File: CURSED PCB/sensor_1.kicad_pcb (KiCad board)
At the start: 4 copper layers, 42 x 40 mm, 85 parts, among them J1 Debugging Connector, J2 Micro_SD_Card, J3 Gecko Connector, J5 G125-MH104M4-04AD000P, U1 STM32G431KBT6, U10 MCP2562, U12 AD5761BRUZ, U2 INA180-A3, U3 MIC94090YC6, U4 SPX3819M5-L-3-3, U5 SPX3819M5-L-3-3, U6 OPA323, U7 MCP3562-E_ST, U8 LT6233, U9 TLV61046ADBVR, Y1 24MHz crystal

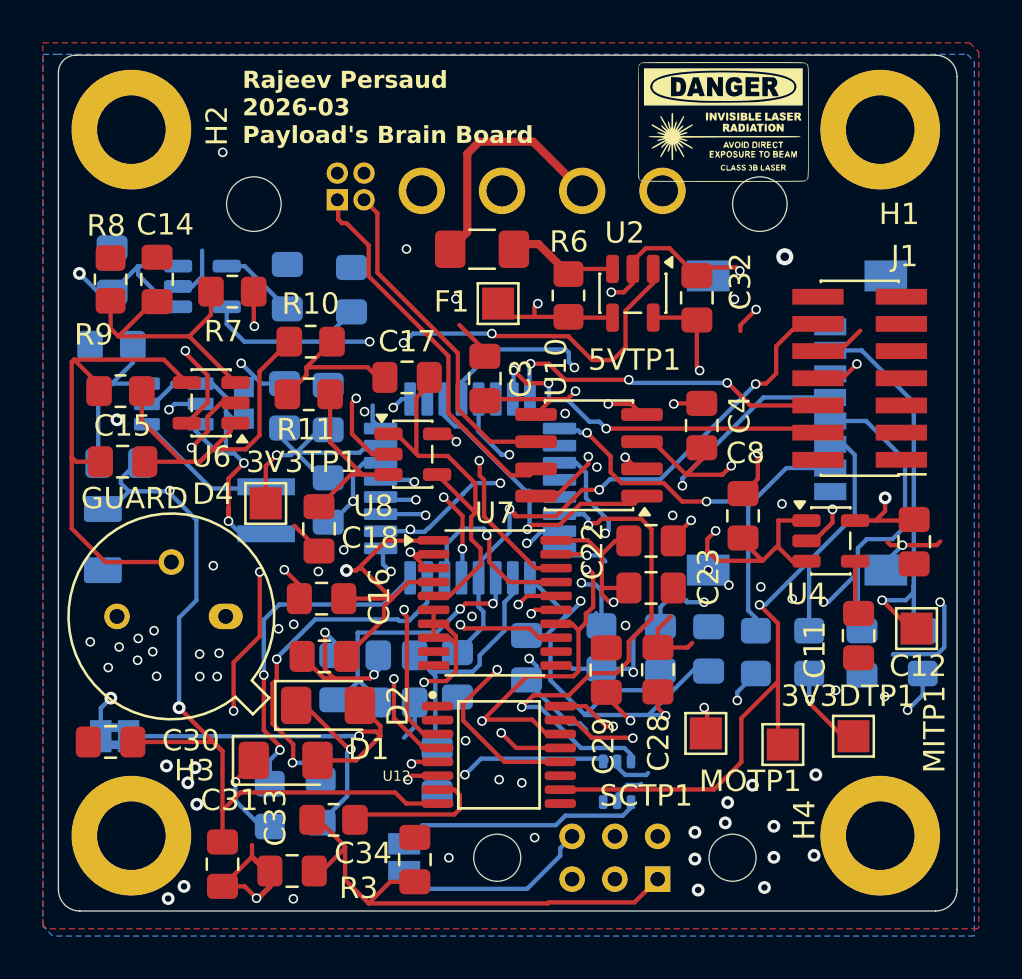
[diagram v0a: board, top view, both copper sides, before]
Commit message: commit for pranav
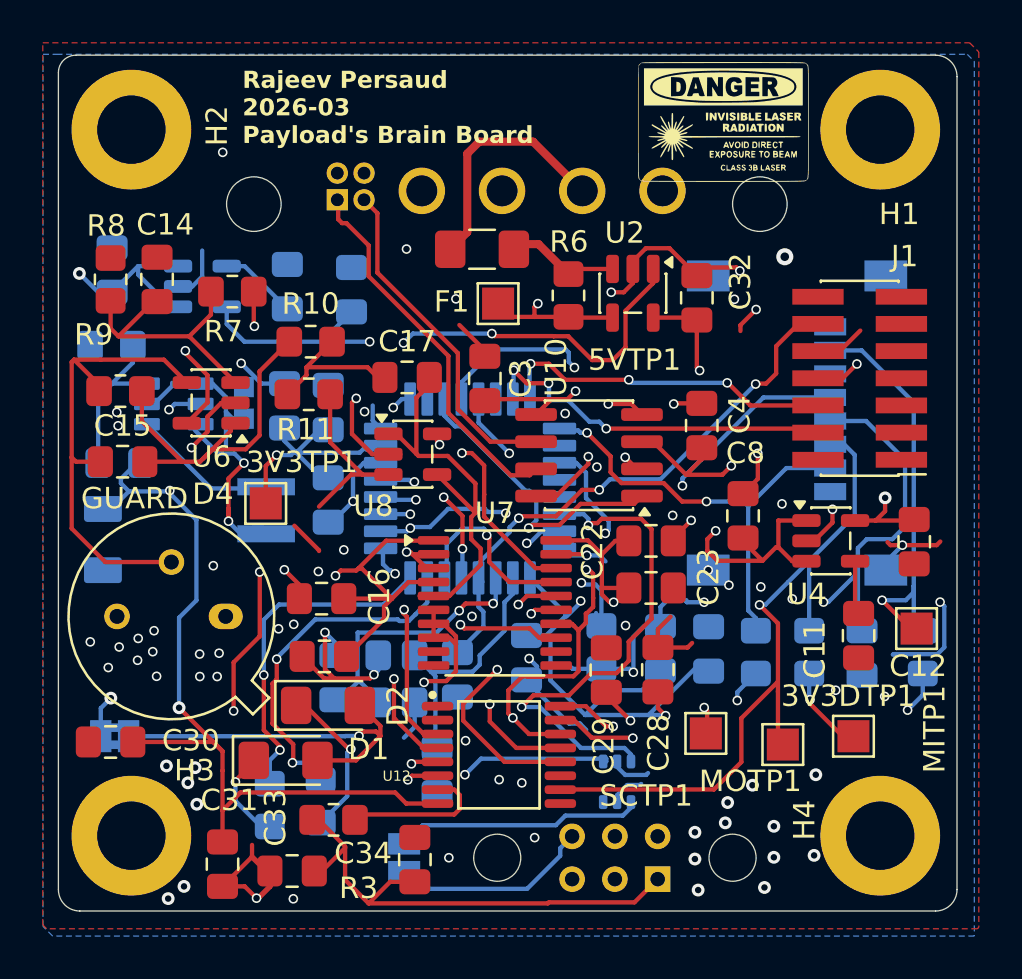
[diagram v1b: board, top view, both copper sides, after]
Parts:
- removed C18: 43nF, Capacitor_SMD:C_0805_2012Metric_Pad1.18x1.45mm_HandSolder
- moved G*** 0.23 mm to (50.3, 40.7)
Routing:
- net +5V: track 108.8 -> 89.9 mm
- net /SCLK: track 56.7 -> 53.4 mm
- net GND: track 119.9 -> 117.1 mm, vias 84 -> 85
- net /MKLKIN: track 12.0 -> 13.7 mm
- net /MCLR: track 27.6 -> 26.5 mm
- net /MCU/CS_DAC: track 18.2 -> 19.1 mm
- net +3.3VA: track 65.4 -> 64.6 mm
